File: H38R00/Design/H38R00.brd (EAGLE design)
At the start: 34.6 x 60 mm, 77 parts, among them P1 HEXABIT_17.32_X2_POWER_ONLY, U1 LM5160DNT, U2 TPS65130RGERT, U3 TPS76433DBVT

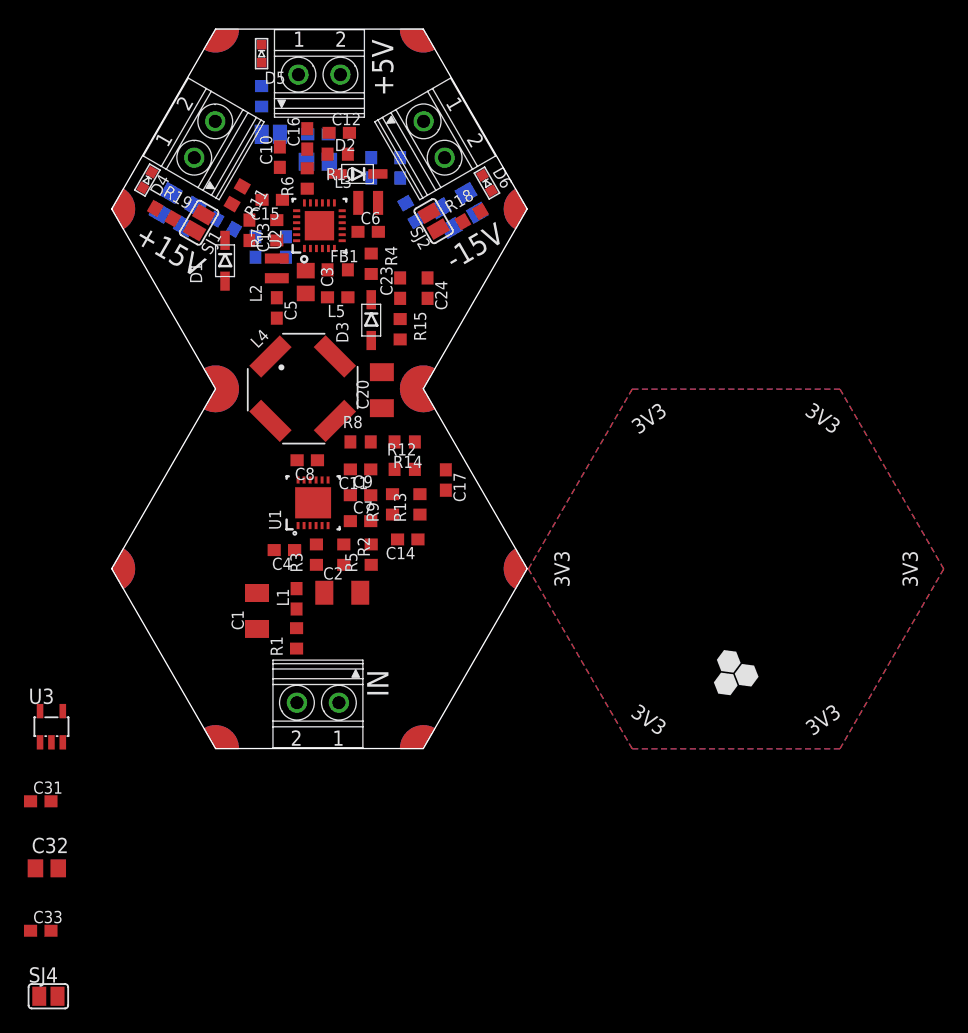
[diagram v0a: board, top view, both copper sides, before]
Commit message: Arranged most silkscreen Added labels
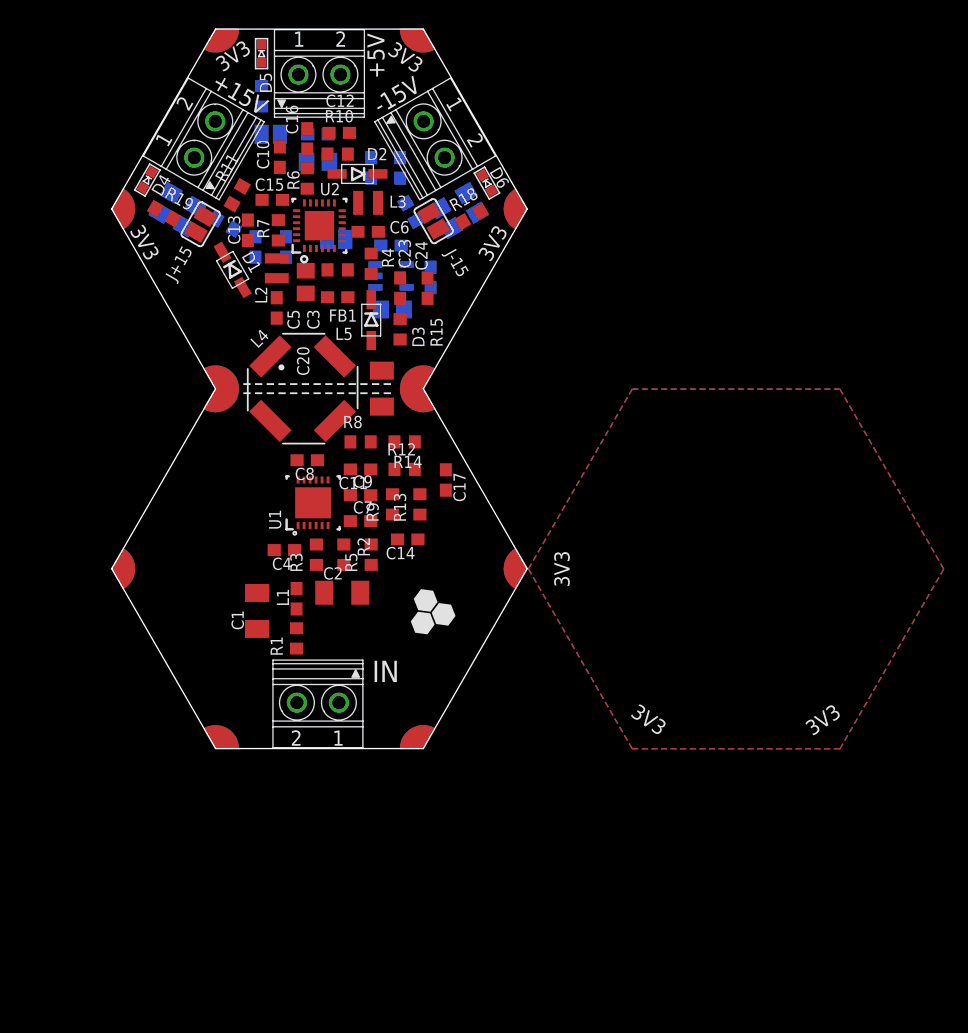
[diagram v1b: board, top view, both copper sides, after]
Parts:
- removed SJ1, SJ4: (no value), jumper:SJ
- added J+15, J3V3: (no value), jumper:SJ
- moved C33 63.4 mm to (42.3, 58.8), flipped to the bottom, turned to 90 degrees
- moved C32 54.8 mm to (39.1, 56.1), flipped to the bottom
- moved C31 54.8 mm to (39.0, 61.5), flipped to the bottom
- moved U3 47.1 mm to (39.0, 58.9), flipped to the bottom, turned to 90 degrees
- moved D1 0.99 mm to (25.8, 59.4), turned to 120 degrees
- moved C13 0.13 mm to (27.1, 62.7)
- moved C20 0.13 mm to (38.2, 49.5)
- moved R7 0.13 mm to (29.6, 62.7)
- renumbered SJ2 to J-15, SJ3 to J5
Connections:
- net +15V: now also J+15.1; no longer SJ1.1
- net +5V: now also J3V3.2; no longer SJ4.2
- net N$31: now also J+15.2; no longer SJ1.2
- net N$36: now also J3V3.1; no longer SJ4.1
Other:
- board text added: "+15V"
- board text added: "+5V"
- board text added: "-15V"
- board text added: "12V .. 36V"
- board text added: "IGND"
